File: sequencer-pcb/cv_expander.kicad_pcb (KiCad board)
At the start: 2 copper layers, 25 x 74 mm, 17 parts, among them J1 Conn_01x20_Male, J10 Gate out, J11 EG out, J12 LFO Out, J13 VCF Out, J14 VCO out, J2 VCA In, J3 VCF In, J4 VCO Lin In, J5 VCO Exp in, J6 LFO in, J7 VCF Aud in, J8 KB CV out, J9 Trig Out

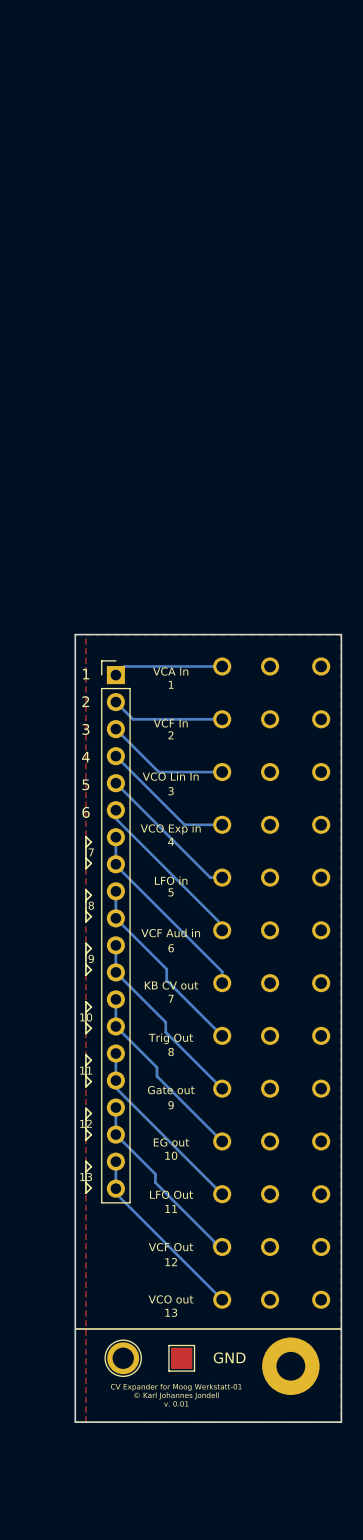
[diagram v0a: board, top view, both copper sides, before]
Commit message: cv expander
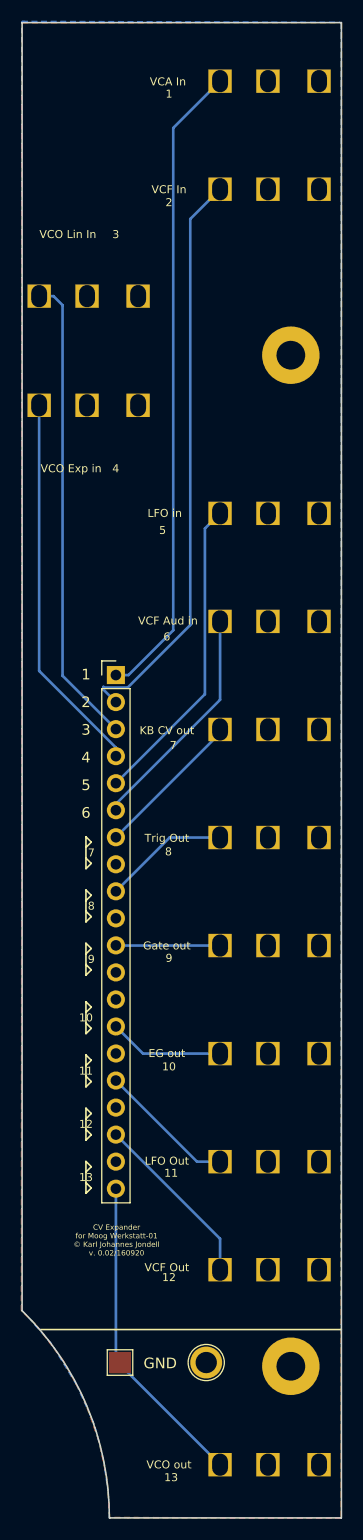
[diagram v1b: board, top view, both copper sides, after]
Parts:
- added GND: MountingHole_GND, MountingHole:MountingHole_2.7mm_M2.5_Pad, F.Cu at (152.2, 52.8)
- moved J2 55.0 mm to (150.0, 27.0)
- moved J3 49.8 mm to (150.0, 37.2)
- moved J4 47.9 mm to (133.0, 47.2)
- moved J5 43.0 mm to (133.0, 57.5)
- moved J6 34.2 mm to (150.0, 67.6)
- moved J7 29.0 mm to (150.0, 77.8)
- moved J8 23.8 mm to (150.0, 87.9)
- moved J9 18.6 mm to (150.0, 98.1)
- moved J14 15.5 mm to (150.0, 157.0)
- moved J10 13.4 mm to (150.0, 108.2)
- moved J11 8.25 mm to (150.0, 118.4)
- moved GND 7.81 mm to (144.3, 147.4)
- moved TP2 5.81 mm to (136.2, 147.4)
- moved J12 3.06 mm to (150.0, 128.5)
- moved J13 2.15 mm to (150.0, 138.7)
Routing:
- net Net-(J1-Pad1): track 10.3 -> 60.6 mm
- net Net-(J1-Pad2): track 10.7 -> 54.6 mm
- net Net-(J1-Pad3): track 11.7 -> 44.5 mm
- net Net-(J1-Pad4): track 12.7 -> 36.0 mm
- net Net-(J1-Pad5): track 13.7 -> 29.4 mm
- net Net-(J1-Pad19): track 17.1 -> 30.0 mm
- net Net-(J1-Pad11): track 17.6 -> 9.80 mm
- net Net-(J1-Pad13): track 17.5 -> 10.8 mm
- net Net-(J1-Pad6): track 15.6 -> 21.8 mm
- net Net-(J1-Pad10): track 17.7 -> 11.9 mm
- net Net-(J1-Pad15): track 17.4 -> 12.9 mm
- net Net-(J1-Pad7): track 17.8 -> 14.2 mm
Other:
- board size 25 x 74 mm -> 30 x 140.5 mm
- board text added: "CV Expander for Moog Werkstatt-01 © Karl Johannes Jondell v. 0.02/160920"
- board text removed: "CV Expander for Moog Werkstatt-01 © Karl Johannes Jondell v. 0.01"
